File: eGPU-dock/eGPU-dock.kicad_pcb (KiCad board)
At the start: 2 copper layers, 40 parts, among them Y1 25MHz

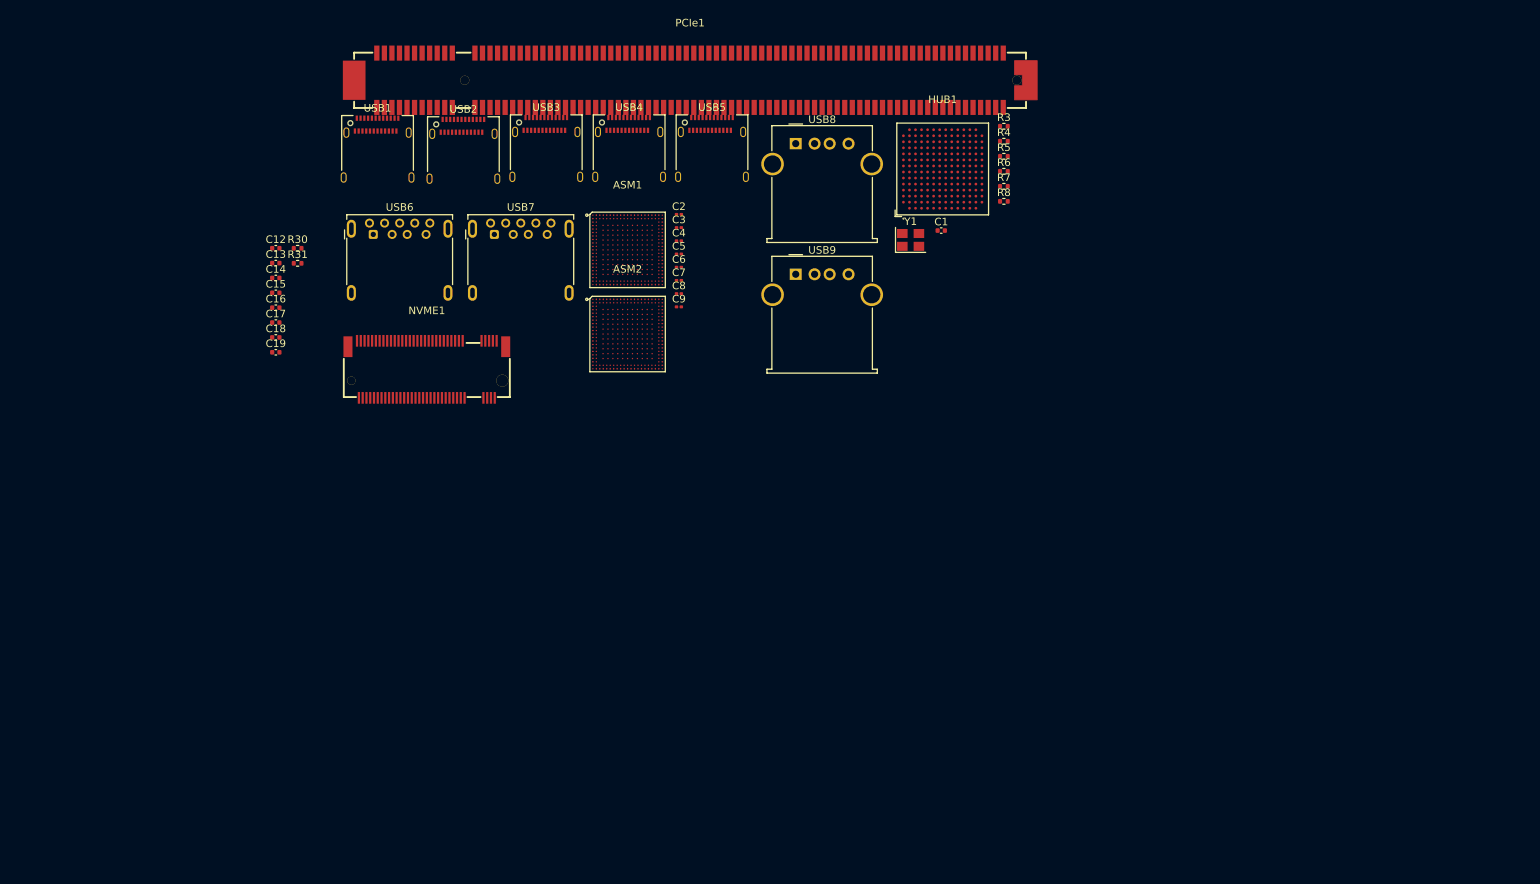
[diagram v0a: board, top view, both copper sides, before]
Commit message: update
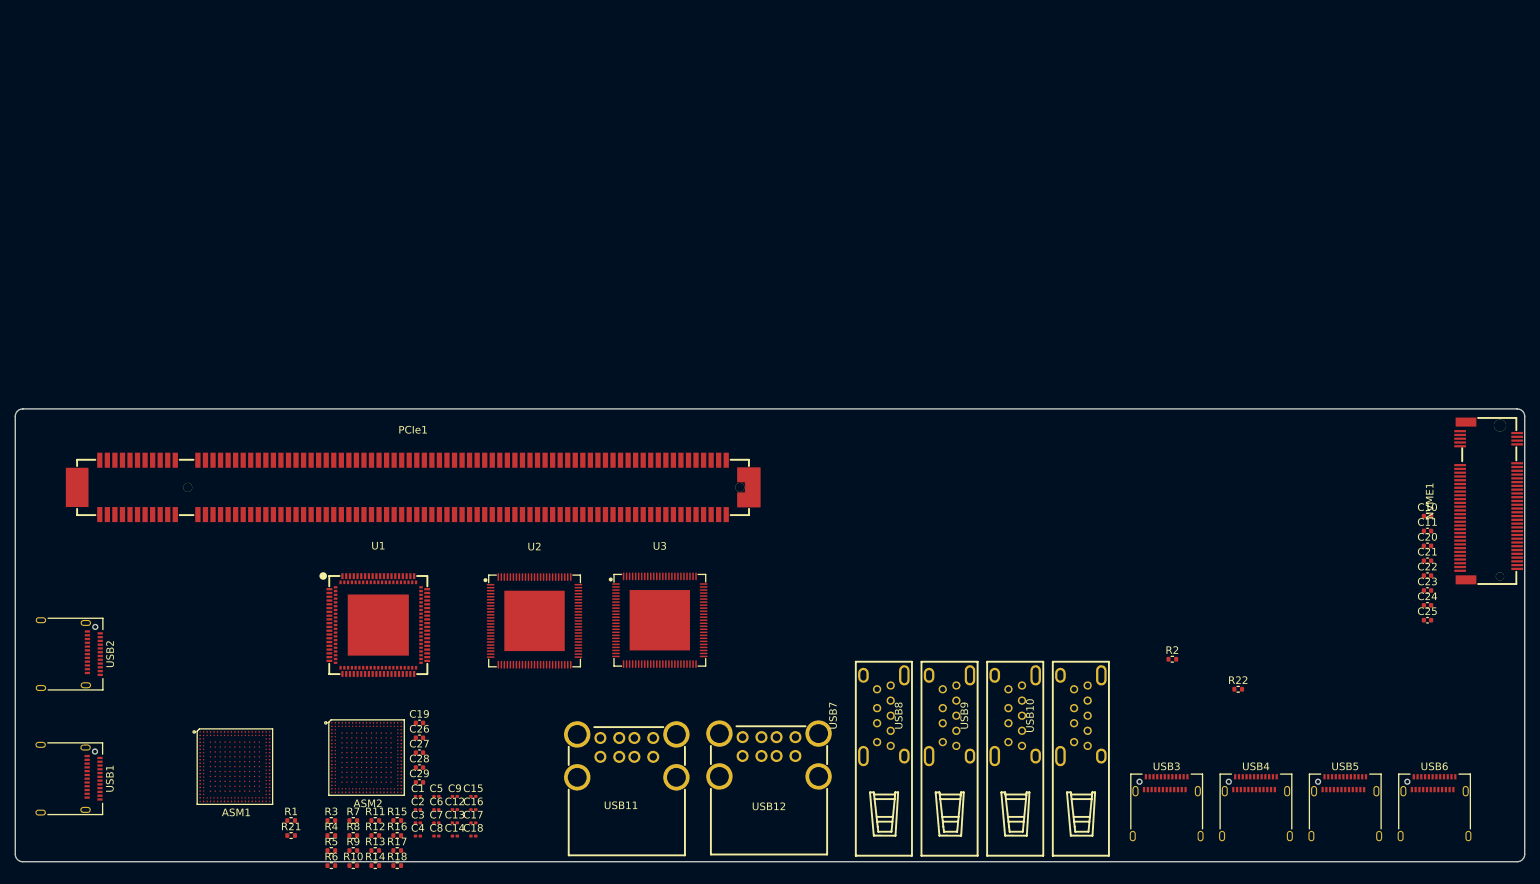
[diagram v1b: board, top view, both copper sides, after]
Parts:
- removed HUB1: CYUSB4347-BZXC, easyeda2kicad:FBGA-192_L12.0-W12.0-P0.80-BL_CY9BF318TBGL-GK7E1
- removed R30, R31: 0Ω, Resistor_SMD:R_0402_1005Metric
- removed Y1: 25MHz, Crystal:Crystal_SMD_3225-4Pin_3.2x2.5mm
- added C10: 0.22u, Capacitor_SMD:C_0402_1005Metric, F.Cu at (237.1, 104.2)
- added C11: 0.22u, Capacitor_SMD:C_0402_1005Metric, F.Cu at (237.1, 106.2)
- added C20: 0.22u, Capacitor_SMD:C_0402_1005Metric, F.Cu at (237.1, 108.2)
- added C21: 0.22u, Capacitor_SMD:C_0402_1005Metric, F.Cu at (237.1, 110.1)
- added C22: 0.22u, Capacitor_SMD:C_0402_1005Metric, F.Cu at (237.1, 112.1)
- added C23: 0.22u, Capacitor_SMD:C_0402_1005Metric, F.Cu at (237.1, 114.1)
- added C24: 0.22u, Capacitor_SMD:C_0402_1005Metric, F.Cu at (237.1, 116.0)
- added C25: 0.22u, Capacitor_SMD:C_0402_1005Metric, F.Cu at (237.1, 118.0)
- added C26: 0.22u, Capacitor_SMD:C_0402_1005Metric, F.Cu at (103.6, 133.6)
- added C27: 0.22u, Capacitor_SMD:C_0402_1005Metric, F.Cu at (103.6, 135.6)
- added C28: 0.22u, Capacitor_SMD:C_0402_1005Metric, F.Cu at (103.6, 137.5)
- added C29: 220p, Capacitor_SMD:C_0402_1005Metric, F.Cu at (103.6, 139.5)
- added R1: 10k, Resistor_SMD:R_0402_1005Metric, F.Cu at (86.5, 144.5)
- added R10: 0Ω, Resistor_SMD:R_0402_1005Metric, F.Cu at (94.8, 150.5)
- added R11: 0Ω, Resistor_SMD:R_0402_1005Metric, F.Cu at (97.7, 144.5)
- added R12: 0Ω, Resistor_SMD:R_0402_1005Metric, F.Cu at (97.7, 146.5)
- added R13: 0Ω, Resistor_SMD:R_0402_1005Metric, F.Cu at (97.7, 148.5)
- added R14: 0Ω, Resistor_SMD:R_0402_1005Metric, F.Cu at (97.7, 150.5)
- added R15: 10k, Resistor_SMD:R_0402_1005Metric, F.Cu at (100.6, 144.5)
- added R16: 10k, Resistor_SMD:R_0402_1005Metric, F.Cu at (100.6, 146.5)
- added R17: 1KΩ, Resistor_SMD:R_0402_1005Metric, F.Cu at (100.6, 148.5)
- added R18: 10KΩ, Resistor_SMD:R_0402_1005Metric, F.Cu at (100.6, 150.5)
- added R2: 0Ω, Resistor_SMD:R_0402_1005Metric, F.Cu at (203.3, 123.2)
- added R21: 10k, Resistor_SMD:R_0402_1005Metric, F.Cu at (86.5, 146.5)
- added R22: 0Ω, Resistor_SMD:R_0402_1005Metric, F.Cu at (212.0, 127.2)
- added R9: 0Ω, Resistor_SMD:R_0402_1005Metric, F.Cu at (94.8, 148.5)
- added U1: PCI11414-I/PMX, easyeda2kicad:QFN-164_L13.0-W13.0-P0.50-TL-EP8.0, F.Cu at (98.1, 118.6)
- added U2: USB7216C/KDX, easyeda2kicad:VQFN-100_L12.0-W12.0-P0.40-TL-EP8.0, F.Cu at (118.8, 118.1)
- added U3: USB7206C-I/KDX, easyeda2kicad:VQFN-100_L12.0-W12.0-P0.40-TL-EP8.0, F.Cu at (135.4, 118.0)
- added USB10: HC-USB3.0-L257-P, easyeda2kicad:USB-3.0-A-TH_HOOYA_USB-303L-L-SU, F.Cu at (191.2, 130.7)
- added USB11: USB-269-BRW, easyeda2kicad:USB-A-TH_USB-269-BRW, F.Cu at (131.0, 136.0)
- added USB12: USB-269-BRW, easyeda2kicad:USB-A-TH_USB-269-BRW, F.Cu at (149.9, 135.9)
- ASM1, ASM2: footprint easyeda2kicad:FCCSP-273_L10.0-W10.0-P0.45-TL -> eGPUlib:ASM2464PDX
- C1: value 10p -> 0.33u; footprint Capacitor_SMD:C_0402_1005Metric -> Capacitor_SMD:C_0201_0603Metric
- C12, C13, C14, C15, C16, C17, C18: value 0.22u -> 0.33u; footprint Capacitor_SMD:C_0402_1005Metric -> Capacitor_SMD:C_0201_0603Metric
- PCIe1: value X1611WVS-164-9TV30 -> PCIexpress_x16
- USB6: value USB3_A -> USB_C_Receptacle; footprint Connector_USB:USB3_A_Molex_48393-001 -> Connector_USB:USB_C_Receptacle_Amphenol_12401610E4-2A
- USB7: value USB3_A -> HC-USB3.0-L257-P; footprint Connector_USB:USB3_A_Molex_48393-001 -> easyeda2kicad:USB-3.0-A-TH_HOOYA_USB-303L-L-SU
- USB8, USB9: value USB_A -> HC-USB3.0-L257-P; footprint Connector_USB:USB_A_Molex_67643_Horizontal -> easyeda2kicad:USB-3.0-A-TH_HOOYA_USB-303L-L-SU
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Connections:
- net /CC1_C renamed /USB4_1_CC1_C
- net /CC2_C renamed /USB4_1_CC2_C
- net /SBU1_C renamed /USB4_1_SBU1_C
- net /SBU2_C renamed /USB4_1_SBU2_C
- net /URX0_C+ renamed /USB4_1_RX0_C+
- net /URX0_C- renamed /USB4_1_RX0_C-
- net /URX1_C+ renamed /USB4_1_RX1_C+
- net /URX1_C- renamed /USB4_1_RX1_C-
- net /USB2_C_D+ renamed /USB4_1_2.0_C_D+
- net /USB2_C_D- renamed /USB4_1_2.0_C_D-
- net /UTX0_C+ renamed /USB4_1_TX0_C+
- net /UTX0_C- renamed /USB4_1_TX0_C-
- net /UTX1_C+ renamed /USB4_1_TX1_C+
- net /UTX1_C- renamed /USB4_1_TX1_C-
- net ActLED1 renamed ASM1_ActLED1
- net ActLED2 renamed ASM1_ActLED2
- net ActLED3 renamed ASM1_ActLED3
- net ActLED4 renamed ASM1_ActLED4
- net CC1 renamed USB4_1_CC1
- net CC2 renamed USB4_1_CC2
- net CLKREQ2# renamed ASM1_CLKREQ2#
- net CLKREQ3# renamed ASM1_CLKREQ3#
- net GPIO1 renamed ASM1_GPIO1
- net GPIO19 renamed ASM1_GPIO19
- net GPIO2 renamed ASM1_GPIO2
- net GPIO20 renamed ASM1_GPIO20
- net GPIO21 renamed ASM1_GPIO21
- net GPIO27 renamed ASM1_GPIO27
- net HDDPC renamed PCIe_HDDPC
- net P1_LED renamed ASM1_P1_LED
- net P2_LED renamed ASM1_P2_LED
- net P3_LED renamed ASM1_P3_LED
- net P4_LED renamed ASM1_P4_LED
- net RST# renamed ASM1_RST#
- net SBU1 renamed USB4_1_SBU1
- net SBU2 renamed USB4_1_SBU2
- net SPI_CLK renamed ASM1_SPI_CLK
- net SPI_CS# renamed ASM1_SPI_CS#
- net SPI_DI renamed ASM1_SPI_DI
- net SPI_DO renamed ASM1_SPI_DO
- net TEST_EN renamed ASM1_TEST_EN
- net UREXT renamed ASM1_UREXT
- net URX0+ renamed USB4_1_RX0+
- net URX0- renamed USB4_1_RX0-
- net URX1+ renamed USB4_1_RX1+
- net URX1- renamed USB4_1_RX1-
- net USB2_D+ renamed USB4_1_2.0_D+
- net USB2_D- renamed USB4_1_2.0_D-
- net UTX0+ renamed USB4_1_TX0+
- net UTX0- renamed USB4_1_TX0-
- net UTX1+ renamed USB4_1_TX1+
- net UTX1- renamed USB4_1_TX1-
- ASM1 pad A13: PE_WAKE# -> ASM1_PE_WAKE#
- ASM1 pad A19: CLKREQ1# -> PCIe_CLKREQ#
- ASM1 pad A20: CLKREQ0# -> ASM1_CLKREQ1#
- ASM1 pad A21: UART_RX -> unconnected-(ASM1B-PRSNT0#/UART_RX-PadA21)
- ASM1 pad AA1: unconnected-(ASM1C-GNDA-PadAA1) -> GNDA
- ASM1 pad AA12: unconnected-(ASM1C-GNDA-PadAA12) -> GNDA
- ASM1 pad AA14: unconnected-(ASM1C-GNDA-PadAA14) -> GNDA
- ASM1 pad AA16: unconnected-(ASM1C-GNDA-PadAA16) -> GNDA
- ASM1 pad AA18: unconnected-(ASM1C-GNDA-PadAA18) -> GNDA
- ASM1 pad AA2: unconnected-(ASM1C-GNDA-PadAA2) -> GNDA
- ASM1 pad AA20: unconnected-(ASM1C-GNDA-PadAA20) -> GNDA
- ASM1 pad AA21: unconnected-(ASM1C-GNDA-PadAA21) -> GNDA
- ASM1 pad AA4: XI -> ASM1_XI
- ASM1 pad AA5: unconnected-(ASM1C-GNDA-PadAA5) -> GNDA
- ASM1 pad AA8: REFCLK+ -> PCIe_REFCLK+
- ASM1 pad AA9: unconnected-(ASM1C-GNDA-PadAA9) -> GNDA
- ASM1 pad B21: UART_TX -> unconnected-(ASM1B-MEMREPAIR/UART_TX-PadB21)
- ASM1 pad D11: unconnected-(ASM1C-GND-PadD11) -> GND
- ASM1 pad D13: unconnected-(ASM1C-VCCH-PadD13) -> +3.3V_LDO
- ASM1 pad D14: unconnected-(ASM1C-VDD-PadD14) -> VDD
- ASM1 pad D16: unconnected-(ASM1C-VDD-PadD16) -> VDD
- ASM1 pad D17: unconnected-(ASM1C-GND-PadD17) -> GND
- ASM1 pad D18: unconnected-(ASM1C-GND-PadD18) -> GND
- ASM1 pad D4: unconnected-(ASM1C-GND-PadD4) -> GND
- ASM1 pad D5: unconnected-(ASM1C-GND-PadD5) -> GND
- ASM1 pad D6: unconnected-(ASM1C-VCCH-PadD6) -> +3.3V_LDO
- ASM1 pad D8: unconnected-(ASM1C-VCCH-PadD8) -> +3.3V_LDO
- ASM1 pad D9: unconnected-(ASM1C-VCCH-PadD9) -> +3.3V_LDO
- ASM1 pad E1: I2C_CLK -> unconnected-(ASM1B-I2C_CLK_P-PadE1)
- ASM1 pad E11: unconnected-(ASM1C-VDD-PadE11) -> VDD
- ASM1 pad E13: unconnected-(ASM1C-VCCH-PadE13) -> +3.3V_LDO
- ASM1 pad E14: unconnected-(ASM1C-VDD-PadE14) -> VDD
- ASM1 pad E16: unconnected-(ASM1C-VDD-PadE16) -> VDD
- ASM1 pad E17: unconnected-(ASM1C-GND-PadE17) -> GND
- ASM1 pad E18: unconnected-(ASM1C-GND-PadE18) -> GND
- ASM1 pad E4: unconnected-(ASM1C-GND-PadE4) -> GND
- ASM1 pad E5: unconnected-(ASM1C-GND-PadE5) -> GND
- ASM1 pad E6: unconnected-(ASM1C-VCCH-PadE6) -> +3.3V_LDO
- ASM1 pad E8: unconnected-(ASM1C-VCCH-PadE8) -> +3.3V_LDO
- ASM1 pad E9: unconnected-(ASM1C-VCCH-PadE9) -> +3.3V_LDO
- ASM1 pad F1: I2C_DATA -> unconnected-(ASM1B-I2C_DATA_P-PadF1)
- ASM1 pad F11: unconnected-(ASM1C-VDD-PadF11) -> VDD
- ASM1 pad F13: unconnected-(ASM1C-VCCH-PadF13) -> +3.3V_LDO
- ASM1 pad F14: unconnected-(ASM1C-VDD-PadF14) -> VDD
- ASM1 pad F16: unconnected-(ASM1C-VDD-PadF16) -> VDD
- ASM1 pad F17: unconnected-(ASM1C-GND-PadF17) -> GND
- ASM1 pad F18: unconnected-(ASM1C-GND-PadF18) -> GND
- ASM1 pad F4: unconnected-(ASM1C-GND-PadF4) -> GND
- ASM1 pad F5: unconnected-(ASM1C-GND-PadF5) -> GND
- ASM1 pad F6: unconnected-(ASM1C-VCCH-PadF6) -> +3.3V_LDO
- ASM1 pad F8: unconnected-(ASM1C-GND-PadF8) -> GND
- ASM1 pad F9: unconnected-(ASM1C-VDD-PadF9) -> VDD
- ASM1 pad G1: VBUS -> ASM1_VBUS
- ASM1 pad G21: PERST0# -> PCIe_PERST0#
- ASM1 pad H11: unconnected-(ASM1C-VDD-PadH11) -> VDD
- ASM1 pad H13: unconnected-(ASM1C-VDD-PadH13) -> VDD
- ASM1 pad H14: unconnected-(ASM1C-VDD-PadH14) -> VDD
- ASM1 pad H16: unconnected-(ASM1C-VDD-PadH16) -> VDD
- ASM1 pad H17: unconnected-(ASM1C-GND-PadH17) -> GND
- ASM1 pad H18: unconnected-(ASM1C-GND-PadH18) -> GND
- ASM1 pad H4: unconnected-(ASM1C-GND-PadH4) -> GND
- ASM1 pad H5: unconnected-(ASM1C-VCCA33-PadH5) -> +3.3VA
- ASM1 pad H6: unconnected-(ASM1C-VCCH-PadH6) -> +3.3V_LDO
- ASM1 pad H8: unconnected-(ASM1C-GND-PadH8) -> GND
- ASM1 pad H9: unconnected-(ASM1C-VDD-PadH9) -> VDD
- ASM1 pad J11: unconnected-(ASM1C-GND-PadJ11) -> GND
- ASM1 pad J13: unconnected-(ASM1C-VDD-PadJ13) -> VDD
- ASM1 pad J14: unconnected-(ASM1C-VDD-PadJ14) -> VDD
- ASM1 pad J16: unconnected-(ASM1C-VDD-PadJ16) -> VDD
- ASM1 pad J17: unconnected-(ASM1C-VDD-PadJ17) -> VDD
- ASM1 pad J18: unconnected-(ASM1C-VDD-PadJ18) -> VDD
- ASM1 pad J20: unconnected-(ASM1C-VDD-PadJ20) -> VDD
- ASM1 pad J21: unconnected-(ASM1C-VDD-PadJ21) -> VDD
- ASM1 pad J4: unconnected-(ASM1C-GND-PadJ4) -> GND
- ASM1 pad J5: unconnected-(ASM1C-GND-PadJ5) -> GND
- ASM1 pad J6: unconnected-(ASM1C-GND-PadJ6) -> GND
- ASM1 pad J8: unconnected-(ASM1C-VDD-PadJ8) -> VDD
- ASM1 pad J9: unconnected-(ASM1C-VDD-PadJ9) -> VDD
- ASM1 pad K2: unconnected-(ASM1C-GND-PadK2) -> GND
- ASM1 pad K20: unconnected-(ASM1C-VDD-PadK20) -> VDD
- ASM1 pad K21: unconnected-(ASM1C-VDD-PadK21) -> VDD
- ASM1 pad L1: unconnected-(ASM1C-GNDA-PadL1) -> GNDA
- ASM1 pad L11: unconnected-(ASM1C-VDD-PadL11) -> VDD
- ASM1 pad L13: unconnected-(ASM1C-GND-PadL13) -> GND
- ASM1 pad L14: unconnected-(ASM1C-VDD-PadL14) -> VDD
- ASM1 pad L16: unconnected-(ASM1C-VCCL-PadL16) -> VCCL
- ASM1 pad L17: unconnected-(ASM1C-VCCL-PadL17) -> VCCL
- ASM1 pad L18: unconnected-(ASM1C-VCCL-PadL18) -> VCCL
- ASM1 pad L2: unconnected-(ASM1C-GNDA-PadL2) -> GNDA
- ASM1 pad L20: unconnected-(ASM1C-VCCL-PadL20) -> VCCL
- ASM1 pad L21: unconnected-(ASM1C-VCCL-PadL21) -> VCCL
- ASM1 pad L4: unconnected-(ASM1C-GNDA-PadL4) -> GNDA
- ASM1 pad L5: unconnected-(ASM1C-GNDA-PadL5) -> GNDA
- ASM1 pad L6: unconnected-(ASM1C-VCCL-PadL6) -> VCCL
- ASM1 pad L8: unconnected-(ASM1C-VDD-PadL8) -> VDD
- ASM1 pad L9: unconnected-(ASM1C-GND-PadL9) -> GND
- ASM1 pad M20: unconnected-(ASM1C-GNDA-PadM20) -> GNDA
- ASM1 pad M21: unconnected-(ASM1C-GNDA-PadM21) -> GNDA
- ASM1 pad N1: unconnected-(ASM1C-GNDA-PadN1) -> GNDA
- ASM1 pad N11: unconnected-(ASM1C-GND-PadN11) -> GND
- ASM1 pad N13: unconnected-(ASM1C-GND-PadN13) -> GND
- ASM1 pad N14: unconnected-(ASM1C-VDD-PadN14) -> VDD
- ASM1 pad N16: unconnected-(ASM1C-VCCL-PadN16) -> VCCL
- ASM1 pad N17: unconnected-(ASM1C-GNDA-PadN17) -> GNDA
- ASM1 pad N18: unconnected-(ASM1C-GNDA-PadN18) -> GNDA
- ASM1 pad N2: unconnected-(ASM1C-GNDA-PadN2) -> GNDA
- ASM1 pad N4: unconnected-(ASM1C-GNDA-PadN4) -> GNDA
- ASM1 pad N5: unconnected-(ASM1C-GNDA-PadN5) -> GNDA
- ASM1 pad N6: unconnected-(ASM1C-VCCL-PadN6) -> VCCL
- ASM1 pad N8: unconnected-(ASM1C-VDD-PadN8) -> VDD
- ASM1 pad N9: unconnected-(ASM1C-GND-PadN9) -> GND
- ASM1 pad P11: unconnected-(ASM1C-GND-PadP11) -> GND
- ASM1 pad P13: unconnected-(ASM1C-VDD-PadP13) -> VDD
- ASM1 pad P14: unconnected-(ASM1C-VDD-PadP14) -> VDD
- ASM1 pad P16: unconnected-(ASM1C-VCCL-PadP16) -> VCCL
- ASM1 pad P17: unconnected-(ASM1C-GNDA-PadP17) -> GNDA
- ASM1 pad P18: unconnected-(ASM1C-GNDA-PadP18) -> GNDA
- ASM1 pad P20: unconnected-(ASM1C-GNDA-PadP20) -> GNDA
- ASM1 pad P21: unconnected-(ASM1C-GNDA-PadP21) -> GNDA
- ASM1 pad P4: unconnected-(ASM1C-GNDA-PadP4) -> GNDA
- ASM1 pad P5: unconnected-(ASM1C-GNDA-PadP5) -> GNDA
- ASM1 pad P6: unconnected-(ASM1C-VCCL-PadP6) -> VCCL
- ASM1 pad P8: unconnected-(ASM1C-VDD-PadP8) -> VDD
- ASM1 pad P9: unconnected-(ASM1C-GND-PadP9) -> GND
- ASM1 pad R1: unconnected-(ASM1C-GNDA-PadR1) -> GNDA
- ASM1 pad R2: unconnected-(ASM1C-GNDA-PadR2) -> GNDA
- ASM1 pad T11: unconnected-(ASM1C-VDD-PadT11) -> VDD
- ASM1 pad T13: unconnected-(ASM1C-VDD-PadT13) -> VDD
- ASM1 pad T14: unconnected-(ASM1C-VDD-PadT14) -> VDD
- ASM1 pad T16: unconnected-(ASM1C-VCCL-PadT16) -> VCCL
- ASM1 pad T17: unconnected-(ASM1C-GNDA-PadT17) -> GNDA
- ASM1 pad T18: unconnected-(ASM1C-GNDA-PadT18) -> GNDA
- ASM1 pad T20: unconnected-(ASM1C-GNDA-PadT20) -> GNDA
- ASM1 pad T21: unconnected-(ASM1C-GNDA-PadT21) -> GNDA
- ASM1 pad T4: unconnected-(ASM1C-GNDA-PadT4) -> GNDA
- ASM1 pad T5: unconnected-(ASM1C-GNDA-PadT5) -> GNDA
- ASM1 pad T6: unconnected-(ASM1C-VCCL-PadT6) -> VCCL
- ASM1 pad T8: unconnected-(ASM1C-VDD-PadT8) -> VDD
- ASM1 pad T9: unconnected-(ASM1C-VDD-PadT9) -> VDD
- ASM1 pad U1: unconnected-(ASM1C-GNDA-PadU1) -> GNDA
- ASM1 pad U11: unconnected-(ASM1C-VCCL-PadU11) -> VCCL
- ASM1 pad U13: unconnected-(ASM1C-VCCL-PadU13) -> VCCL
- ASM1 pad U14: unconnected-(ASM1C-VCCL-PadU14) -> VCCL
- ASM1 pad U16: unconnected-(ASM1C-VCCL-PadU16) -> VCCL
- ASM1 pad U17: unconnected-(ASM1C-GNDA-PadU17) -> GNDA
- ASM1 pad U18: unconnected-(ASM1C-GNDA-PadU18) -> GNDA
- ASM1 pad U2: unconnected-(ASM1C-GNDA-PadU2) -> GNDA
- ASM1 pad U4: unconnected-(ASM1C-GNDA-PadU4) -> GNDA
- ASM1 pad U5: unconnected-(ASM1C-GNDA-PadU5) -> GNDA
- ASM1 pad U6: unconnected-(ASM1C-VCCL-PadU6) -> VCCL
- ASM1 pad U8: unconnected-(ASM1C-VDD-PadU8) -> VDD
- ASM1 pad U9: unconnected-(ASM1C-VDD-PadU9) -> VDD
- ASM1 pad V11: unconnected-(ASM1C-GNDA-PadV11) -> GNDA
- ASM1 pad V13: unconnected-(ASM1C-GNDA-PadV13) -> GNDA
- ASM1 pad V14: unconnected-(ASM1C-GNDA-PadV14) -> GNDA
- ASM1 pad V16: unconnected-(ASM1C-GNDA-PadV16) -> GNDA
- ASM1 pad V17: unconnected-(ASM1C-GNDA-PadV17) -> GNDA
- ASM1 pad V18: unconnected-(ASM1C-GNDA-PadV18) -> GNDA
- ASM1 pad V20: unconnected-(ASM1C-GNDA-PadV20) -> GNDA
- ASM1 pad V21: unconnected-(ASM1C-GNDA-PadV21) -> GNDA
- ASM1 pad V4: unconnected-(ASM1C-GNDA-PadV4) -> GNDA
- ASM1 pad V5: unconnected-(ASM1C-GNDA-PadV5) -> GNDA
- ASM1 pad V6: unconnected-(ASM1C-GNDA-PadV6) -> GNDA
- ASM1 pad V8: unconnected-(ASM1C-GNDA-PadV8) -> GNDA
- ASM1 pad V9: unconnected-(ASM1C-GNDA-PadV9) -> GNDA
- ASM1 pad W1: unconnected-(ASM1C-GNDA-PadW1) -> GNDA
- ASM1 pad W2: unconnected-(ASM1C-GNDA-PadW2) -> GNDA
- ASM1 pad Y12: unconnected-(ASM1C-GNDA-PadY12) -> GNDA
- ASM1 pad Y14: unconnected-(ASM1C-GNDA-PadY14) -> GNDA
- ASM1 pad Y16: unconnected-(ASM1C-GNDA-PadY16) -> GNDA
- ASM1 pad Y18: unconnected-(ASM1C-GNDA-PadY18) -> GNDA
- ASM1 pad Y20: unconnected-(ASM1C-GNDA-PadY20) -> GNDA
- ASM1 pad Y21: unconnected-(ASM1C-GNDA-PadY21) -> GNDA
- ASM1 pad Y3: unconnected-(ASM1C-GNDA-PadY3) -> GNDA
- ASM1 pad Y4: XO -> ASM1_XO
- ASM1 pad Y5: unconnected-(ASM1C-GNDA-PadY5) -> GNDA
- ASM1 pad Y8: REFCLK- -> PCIe_REFCLK-
- ASM1 pad Y9: unconnected-(ASM1C-GNDA-PadY9) -> GNDA
- ASM2 pad A1: unconnected-(ASM2A-GPIO3-PadA1) -> ASM2_ActLED2
- ASM2 pad A10: unconnected-(ASM2A-GPIO19-PadA10) -> ASM2_GPIO19
- ASM2 pad A11: unconnected-(ASM2A-GPIO20-PadA11) -> ASM2_GPIO20
- ASM2 pad A12: unconnected-(ASM2A-GPIO21-PadA12) -> ASM2_GPIO21
- ASM2 pad A13: unconnected-(ASM2A-GPIO22-PadA13) -> ASM2_PE_WAKE#
- ASM2 pad A14: unconnected-(ASM2A-GPIO23-PadA14) -> ASM2_CLKREQ2#
- ASM2 pad A15: unconnected-(ASM2A-GPIO24-PadA15) -> ASM2_CLKREQ3#
- ASM2 pad A16: unconnected-(ASM2A-GPIO25-PadA16) -> ASM2_ActLED3
- ASM2 pad A17: unconnected-(ASM2A-GPIO26-PadA17) -> ASM2_ActLED4
- ASM2 pad A18: unconnected-(ASM2A-GPIO27-PadA18) -> ASM2_GPIO27
- ASM2 pad A19: unconnected-(ASM2A-GPIO8-PadA19) -> M.2_CLKREQ#
- ASM2 pad A2: unconnected-(ASM2A-SPI_CS#-PadA2) -> ASM2_SPI_CS#
- ASM2 pad A20: unconnected-(ASM2A-GPIO14-PadA20) -> SW_CLKREQ#
- ASM2 pad A3: unconnected-(ASM2A-SPI_DO-PadA3) -> ASM2_SPI_DO
- ASM2 pad A4: unconnected-(ASM2A-SPI_DI-PadA4) -> ASM2_SPI_DI
- ASM2 pad A5: unconnected-(ASM2A-SPI_CLK-PadA5) -> ASM2_SPI_CLK
- ASM2 pad A6: unconnected-(ASM2A-GPIO15-PadA6) -> ASM2_P1_LED
- ASM2 pad A7: unconnected-(ASM2A-GPIO16-PadA7) -> ASM2_P2_LED
- ASM2 pad A8: unconnected-(ASM2A-GPIO17-PadA8) -> ASM2_P3_LED
- ASM2 pad A9: unconnected-(ASM2A-GPIO18-PadA9) -> ASM2_P4_LED
- ASM2 pad AA1: unconnected-(ASM2C-GNDA-PadAA1) -> GNDA
- ASM2 pad AA10: unconnected-(ASM2B-NC-PadAA10) -> SW_REFCLK+
- ASM2 pad AA12: unconnected-(ASM2C-GNDA-PadAA12) -> GNDA
- ASM2 pad AA13: unconnected-(ASM2A-PRXP3-PadAA13) -> SW_RX1+
- ASM2 pad AA14: unconnected-(ASM2C-GNDA-PadAA14) -> GNDA
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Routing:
- added copper zone on In1.Cu, net GND
- added copper zone on In10.Cu, net GND
- added copper zone on In3.Cu, net GND
- added copper zone on In6.Cu, net GND
- added copper zone on In8.Cu, net GND
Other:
- board outline added: 200 x 60 mm
- copper layers 2 -> 16

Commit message: masive schamatic update
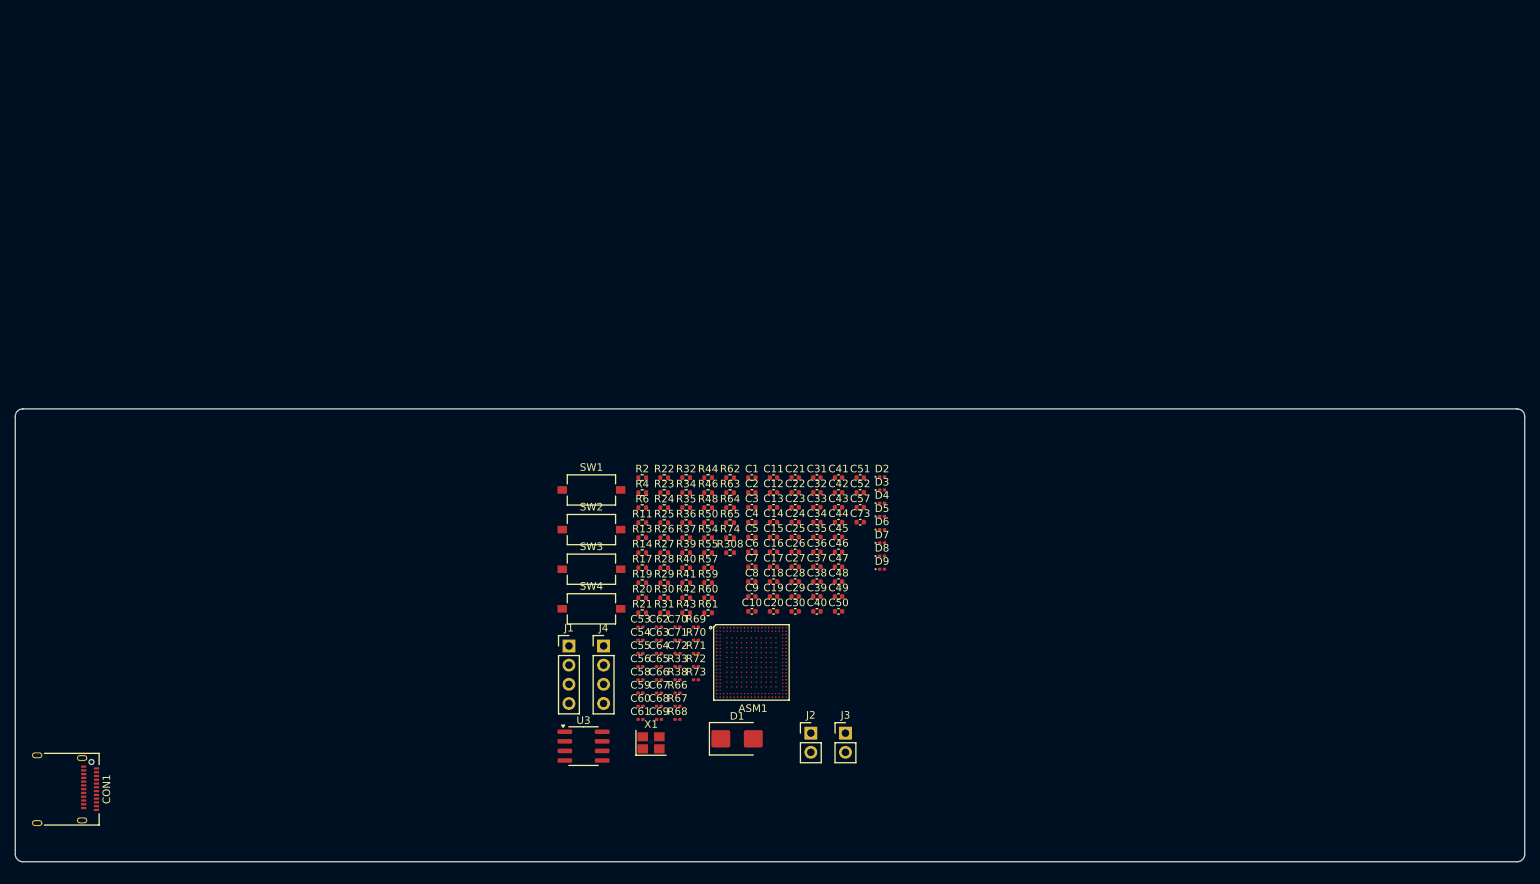
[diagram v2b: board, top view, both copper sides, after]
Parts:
- removed ASM2: ~, eGPUlib:ASM2464PDX
- removed NVME1: AS0BC21-S40BM-7H, easyeda2kicad:CONN-SMD_AS0BC21-S40BM-7H
- removed PCIe1: PCIexpress_x16, easyeda2kicad:CONN-SMD_164P-P1.00_X1611WVS-164-9TV30
- removed R1, R15, R16: 10k, Resistor_SMD:R_0402_1005Metric
- removed R10, R12, R3, R5, R7, R8, R9: 0Ω, Resistor_SMD:R_0402_1005Metric
- removed R18: 10KΩ, Resistor_SMD:R_0402_1005Metric
- removed U1: PCI11414-I/PMX, easyeda2kicad:QFN-164_L13.0-W13.0-P0.50-TL-EP8.0
- removed U2: USB7216C/KDX, easyeda2kicad:VQFN-100_L12.0-W12.0-P0.40-TL-EP8.0
- removed USB1, USB2, USB3, USB4, USB5, USB6: USB_C_Receptacle, Connector_USB:USB_C_Receptacle_Amphenol_12401610E4-2A
- removed USB10, USB7, USB8, USB9: HC-USB3.0-L257-P, easyeda2kicad:USB-3.0-A-TH_HOOYA_USB-303L-L-SU
- removed USB11, USB12: USB-269-BRW, easyeda2kicad:USB-A-TH_USB-269-BRW
- added C30: 0.22UF/10V, Capacitor_SMD:C_0402_1005Metric, F.Cu at (153.3, 116.8)
- added C31: 0.22UF/10V, Capacitor_SMD:C_0402_1005Metric, F.Cu at (156.2, 99.1)
- added C32: 0.22UF/6.3V, Capacitor_SMD:C_0402_1005Metric, F.Cu at (156.2, 101.1)
- added C33: 0.22UF/6.3V, Capacitor_SMD:C_0402_1005Metric, F.Cu at (156.2, 103.0)
- added C34: 0.22UF/10V, Capacitor_SMD:C_0402_1005Metric, F.Cu at (156.2, 105.0)
- added C35: 0.22UF/10V, Capacitor_SMD:C_0402_1005Metric, F.Cu at (156.2, 107.0)
- added C36: 0.22UF/6.3V, Capacitor_SMD:C_0402_1005Metric, F.Cu at (156.2, 109.0)
- added C37: 0.22UF/6.3V, Capacitor_SMD:C_0402_1005Metric, F.Cu at (156.2, 110.9)
- added C38: 10PF/50V, Capacitor_SMD:C_0402_1005Metric, F.Cu at (156.2, 112.9)
- added C39: 0.22UF/10V, Capacitor_SMD:C_0402_1005Metric, F.Cu at (156.2, 114.9)
- added C40: 0.22UF/6.3V, Capacitor_SMD:C_0402_1005Metric, F.Cu at (156.2, 116.8)
- added C41: 0.22UF/6.3V, Capacitor_SMD:C_0402_1005Metric, F.Cu at (159.1, 99.1)
- added C42: 0.22UF/6.3V, Capacitor_SMD:C_0402_1005Metric, F.Cu at (159.1, 101.1)
- added C43: 0.22UF/6.3V, Capacitor_SMD:C_0402_1005Metric, F.Cu at (159.1, 103.0)
- added C44: 0.22UF/6.3V, Capacitor_SMD:C_0402_1005Metric, F.Cu at (159.1, 105.0)
- added C45: 0.22UF/6.3V, Capacitor_SMD:C_0402_1005Metric, F.Cu at (159.1, 107.0)
- added C46: 0.22UF/6.3V, Capacitor_SMD:C_0402_1005Metric, F.Cu at (159.1, 109.0)
- added C47: 0.22UF/16V, Capacitor_SMD:C_0402_1005Metric, F.Cu at (159.1, 110.9)
- added C48: 0.22UF/16V, Capacitor_SMD:C_0402_1005Metric, F.Cu at (159.1, 112.9)
- added C49: 1UF/10V, Capacitor_SMD:C_0402_1005Metric, F.Cu at (159.1, 114.9)
- added C50: 1UF/10V, Capacitor_SMD:C_0402_1005Metric, F.Cu at (159.1, 116.8)
- added C51: 1UF/10V, Capacitor_SMD:C_0402_1005Metric, F.Cu at (161.9, 99.1)
- added C52: 1UF/10V, Capacitor_SMD:C_0402_1005Metric, F.Cu at (161.9, 101.1)
- added C53: 220PF/50V, Capacitor_SMD:C_0201_0603Metric, F.Cu at (132.8, 118.9)
- added C54: 220PF/50V, Capacitor_SMD:C_0201_0603Metric, F.Cu at (132.8, 120.6)
- added C55: 0.1UF/25V, Capacitor_SMD:C_0201_0603Metric, F.Cu at (132.8, 122.4)
- added C56: 0.1UF/25V, Capacitor_SMD:C_0201_0603Metric, F.Cu at (132.8, 124.1)
- added C57: 0.1UF/16V, Capacitor_SMD:C_0402_1005Metric, F.Cu at (161.9, 103.0)
- added C58: 0.1UF/25V, Capacitor_SMD:C_0201_0603Metric, F.Cu at (132.8, 125.9)
- added C59: 0.1UF/25V, Capacitor_SMD:C_0201_0603Metric, F.Cu at (132.8, 127.6)
- added C60: 0.1UF/25V, Capacitor_SMD:C_0201_0603Metric, F.Cu at (132.8, 129.4)
- added C61: 0.1UF/25V, Capacitor_SMD:C_0201_0603Metric, F.Cu at (132.8, 131.1)
- added C62: 0.33UF/25V, Capacitor_SMD:C_0201_0603Metric, F.Cu at (135.3, 118.9)
- added C63: 0.33UF/25V, Capacitor_SMD:C_0201_0603Metric, F.Cu at (135.3, 120.6)
- added C64: 0.33UF/25V, Capacitor_SMD:C_0201_0603Metric, F.Cu at (135.3, 122.4)
- added C65: 0.33UF/25V, Capacitor_SMD:C_0201_0603Metric, F.Cu at (135.3, 124.1)
- added C66: 0.1UF/16V, Capacitor_SMD:C_0201_0603Metric, F.Cu at (135.3, 125.9)
- added C67: 0.1UF/16V, Capacitor_SMD:C_0201_0603Metric, F.Cu at (135.3, 127.6)
- added C68: 1UF/16V, Capacitor_SMD:C_0201_0603Metric, F.Cu at (135.3, 129.4)
- added C69: 0.33UF/25V, Capacitor_SMD:C_0201_0603Metric, F.Cu at (135.3, 131.1)
- added C70: 0.33UF/25V, Capacitor_SMD:C_0201_0603Metric, F.Cu at (137.7, 118.9)
- added C71: 0.33UF/25V, Capacitor_SMD:C_0201_0603Metric, F.Cu at (137.7, 120.6)
- added C72: 0.33UF/25V, Capacitor_SMD:C_0201_0603Metric, F.Cu at (137.7, 122.4)
- added C73: 0.1UF/16V, Capacitor_SMD:C_0402_1005Metric, F.Cu at (161.9, 105.0)
- added CON1: USB_C_Plug, Connector_USB:USB_C_Receptacle_Amphenol_12401610E4-2A, F.Cu at (55.7, 140.4)
- added D1: SR34, Diode_SMD:D_SMB, F.Cu at (145.6, 133.7)
- added D2: ESD150, Diode_SMD:D_0201_0603Metric, F.Cu at (164.8, 99.0)
- added D3: ESD150, Diode_SMD:D_0201_0603Metric, F.Cu at (164.8, 100.7)
- added D4: ESD150, Diode_SMD:D_0201_0603Metric, F.Cu at (164.8, 102.5)
- added D5: ESD150, Diode_SMD:D_0201_0603Metric, F.Cu at (164.8, 104.2)
- added D6: ESD150, Diode_SMD:D_0201_0603Metric, F.Cu at (164.8, 106.0)
- added D7: ESD150, Diode_SMD:D_0201_0603Metric, F.Cu at (164.8, 107.7)
- added D8: ESD150, Diode_SMD:D_0201_0603Metric, F.Cu at (164.8, 109.5)
- added D9: ESD150, Diode_SMD:D_0201_0603Metric, F.Cu at (164.8, 111.2)
- added J1: Conn_01x04, Connector_PinHeader_2.54mm:PinHeader_1x04_P2.54mm_Vertical, F.Cu at (123.4, 121.4)
- added J2: Conn_01x02, Connector_PinHeader_2.54mm:PinHeader_1x02_P2.54mm_Vertical, F.Cu at (155.4, 133.0)
- added J3: Conn_01x02, Connector_PinHeader_2.54mm:PinHeader_1x02_P2.54mm_Vertical, F.Cu at (160.0, 133.0)
- added J4: Conn_01x04, Connector_PinHeader_2.54mm:PinHeader_1x04_P2.54mm_Vertical, F.Cu at (128.0, 121.4)
- added R19: 0Ω, Resistor_SMD:R_0402_1005Metric, F.Cu at (133.1, 113.0)
- added R20: 100KΩ, Resistor_SMD:R_0402_1005Metric, F.Cu at (133.1, 115.0)
- added R23: 1KΩ, Resistor_SMD:R_0402_1005Metric, F.Cu at (136.0, 101.1)
- added R24: 100KΩ, Resistor_SMD:R_0402_1005Metric, F.Cu at (136.0, 103.1)
- added R25: 0Ω, Resistor_SMD:R_0402_1005Metric, F.Cu at (136.0, 105.1)
- added R26: 0Ω, Resistor_SMD:R_0402_1005Metric, F.Cu at (136.0, 107.1)
- added R27: 100KΩ, Resistor_SMD:R_0402_1005Metric, F.Cu at (136.0, 109.1)
- added R28: 100KΩ, Resistor_SMD:R_0402_1005Metric, F.Cu at (136.0, 111.0)
- added R29: 0Ω, Resistor_SMD:R_0402_1005Metric, F.Cu at (136.0, 113.0)
- added R30: 100KΩ, Resistor_SMD:R_0402_1005Metric, F.Cu at (136.0, 115.0)
- added R308: 0Ω, Resistor_SMD:R_0402_1005Metric, F.Cu at (144.7, 109.1)
- added R31: 0Ω, Resistor_SMD:R_0402_1005Metric, F.Cu at (136.0, 117.0)
- added R32: 0Ω, Resistor_SMD:R_0402_1005Metric, F.Cu at (138.9, 99.1)
- added R33: 0Ω, Resistor_SMD:R_0201_0603Metric, F.Cu at (137.7, 124.1)
- added R34: 0Ω, Resistor_SMD:R_0402_1005Metric, F.Cu at (138.9, 101.1)
- added R35: 1KΩ, Resistor_SMD:R_0402_1005Metric, F.Cu at (138.9, 103.1)
- added R36: 0Ω, Resistor_SMD:R_0402_1005Metric, F.Cu at (138.9, 105.1)
- added R37: 0Ω, Resistor_SMD:R_0402_1005Metric, F.Cu at (138.9, 107.1)
- added R38: 0Ω, Resistor_SMD:R_0201_0603Metric, F.Cu at (137.7, 125.9)
- added R39: 2MΩ, Resistor_SMD:R_0402_1005Metric, F.Cu at (138.9, 109.1)
- added R40: 2MΩ, Resistor_SMD:R_0402_1005Metric, F.Cu at (138.9, 111.0)
- added R41: 0Ω, Resistor_SMD:R_0402_1005Metric, F.Cu at (138.9, 113.0)
- added R42: 12.1KΩ, Resistor_SMD:R_0402_1005Metric, F.Cu at (138.9, 115.0)
- added R43: 4.7KΩ, Resistor_SMD:R_0402_1005Metric, F.Cu at (138.9, 117.0)
- added R44: 4.7KΩ, Resistor_SMD:R_0402_1005Metric, F.Cu at (141.8, 99.1)
- added R46: 4.7KΩ, Resistor_SMD:R_0402_1005Metric, F.Cu at (141.8, 101.1)
- added R48: 4.7KΩ, Resistor_SMD:R_0402_1005Metric, F.Cu at (141.8, 103.1)
- added R50: 4.7KΩ, Resistor_SMD:R_0402_1005Metric, F.Cu at (141.8, 105.1)
- added R54: 0Ω, Resistor_SMD:R_0402_1005Metric, F.Cu at (141.8, 107.1)
- added R55: 0Ω, Resistor_SMD:R_0402_1005Metric, F.Cu at (141.8, 109.1)
- added R57: 4.7KΩ, Resistor_SMD:R_0402_1005Metric, F.Cu at (141.8, 111.0)
- added R59: 0Ω, Resistor_SMD:R_0402_1005Metric, F.Cu at (141.8, 113.0)
- added R60: 10KΩ, Resistor_SMD:R_0402_1005Metric, F.Cu at (141.8, 115.0)
- added R61: 4.7KΩ, Resistor_SMD:R_0402_1005Metric, F.Cu at (141.8, 117.0)
- added R62: 4.7KΩ, Resistor_SMD:R_0402_1005Metric, F.Cu at (144.7, 99.1)
- added R63: 0Ω, Resistor_SMD:R_0402_1005Metric, F.Cu at (144.7, 101.1)
- added R64: 0Ω, Resistor_SMD:R_0402_1005Metric, F.Cu at (144.7, 103.1)
- added R65: 0Ω, Resistor_SMD:R_0402_1005Metric, F.Cu at (144.7, 105.1)
- added R66: 220KΩ, Resistor_SMD:R_0201_0603Metric, F.Cu at (137.7, 127.6)
- added R67: 220KΩ, Resistor_SMD:R_0201_0603Metric, F.Cu at (137.7, 129.4)
- added R68: 220KΩ, Resistor_SMD:R_0201_0603Metric, F.Cu at (137.7, 131.1)
- added R69: 220KΩ, Resistor_SMD:R_0201_0603Metric, F.Cu at (140.2, 118.9)
- added R70: 220KΩ, Resistor_SMD:R_0201_0603Metric, F.Cu at (140.2, 120.6)
- added R71: 220KΩ, Resistor_SMD:R_0201_0603Metric, F.Cu at (140.2, 122.4)
- added R72: 220KΩ, Resistor_SMD:R_0201_0603Metric, F.Cu at (140.2, 124.1)
- added R73: 220KΩ, Resistor_SMD:R_0201_0603Metric, F.Cu at (140.2, 125.9)
- added R74: 0Ω, Resistor_SMD:R_0402_1005Metric, F.Cu at (144.7, 107.1)
- added SW1: SW_Push, Button_Switch_SMD:SW_Tactile_SPST_NO_Straight_CK_PTS636Sx25SMTRLFS, F.Cu at (126.3, 100.7)
- added SW2: SW_Push, Button_Switch_SMD:SW_Tactile_SPST_NO_Straight_CK_PTS636Sx25SMTRLFS, F.Cu at (126.3, 106.0)
- added SW3: SW_Push, Button_Switch_SMD:SW_Tactile_SPST_NO_Straight_CK_PTS636Sx25SMTRLFS, F.Cu at (126.3, 111.2)
- added SW4: SW_Push, Button_Switch_SMD:SW_Tactile_SPST_NO_Straight_CK_PTS636Sx25SMTRLFS, F.Cu at (126.3, 116.5)
- added X1: 25 Mhz, Crystal:Crystal_SMD_Abracon_ABM8AIG-4Pin_3.2x2.5mm, F.Cu at (134.2, 134.2)
- C1, C15, C16, C17, C2, C3, C9: value 0.33u -> 2.2UF/6.3V; footprint Capacitor_SMD:C_0201_0603Metric -> Capacitor_SMD:C_0402_1005Metric
- C10, C11: value 0.22u -> 2.2UF/6.3V
- C12, C13, C14, C18, C4, C5, C6: value 0.33u -> 10UF/6.3V; footprint Capacitor_SMD:C_0201_0603Metric -> Capacitor_SMD:C_0402_1005Metric
- C19, C20, C21: value 0.22u -> 10UF/6.3V
- C22, C24, C25, C28: value 0.22u -> 0.22UF/6.3V
- C23, C26, C27: value 0.22u -> 0.22UF/10V
- C29: value 220p -> 0.22UF/6.3V
- C7: value 0.33u -> 22UF/6.3V; footprint Capacitor_SMD:C_0201_0603Metric -> Capacitor_SMD:C_0402_1005Metric
- C8: value 0.33u -> 0.22UF/10V; footprint Capacitor_SMD:C_0201_0603Metric -> Capacitor_SMD:C_0402_1005Metric
- R13: value 0Ω -> 4.7KΩ
- R14, R22: value 0Ω -> 1KΩ
- R17: value 1KΩ -> 0Ω
- R2: value 0Ω -> 20Ω
- R21: value 10k -> 100KΩ
- R6: value 0Ω -> 100KΩ
- U3: value USB7206C-I/KDX -> W25X20CLSN; footprint easyeda2kicad:VQFN-100_L12.0-W12.0-P0.40-TL-EP8.0 -> Package_SO:SOIC-8_3.9x4.9mm_P1.27mm
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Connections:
- net ASM1_ActLED3 renamed GPIO25
- net ASM1_ActLED4 renamed GPIO26
- net ASM1_CLKREQ1# renamed GPIO14
- net ASM1_CLKREQ2# renamed GPIO23
- net ASM1_CLKREQ3# renamed GPIO24
- net ASM1_GPIO19 renamed GPIO19
- net ASM1_GPIO20 renamed GPIO20
- net ASM1_GPIO21 renamed GPIO21
- net ASM1_P1_LED renamed P1_LED
- net ASM1_P2_LED renamed P2_LED
- net ASM1_P3_LED renamed P3_LED
- net ASM1_P4_LED renamed P4_LED
- net ASM1_XI renamed X1
- ASM1 pad A1: ASM1_ActLED2 -> GPIO3
- ASM1 pad A13: ASM1_PE_WAKE# -> GPIO22
- ASM1 pad A18: ASM1_GPIO27 -> GPIO27
- ASM1 pad A19: PCIe_CLKREQ# -> GPIO8
- ASM1 pad A2: ASM1_SPI_CS# -> SPI_CS#
- ASM1 pad A21: unconnected-(ASM1B-PRSNT0#/UART_RX-PadA21) -> UART_RX
- ASM1 pad A3: ASM1_SPI_DO -> SPI_DO
- ASM1 pad A4: ASM1_SPI_DI -> SPI_DI
- ASM1 pad A5: ASM1_SPI_CLK -> SPI_CLK
- ASM1 pad AA1: GNDA -> GND
- ASM1 pad AA10: unconnected-(ASM1A-NC/REFCLKP2-PadAA10) -> REFCLK2+
- ASM1 pad AA11: unconnected-(ASM1A-NC/REFCLKP1-PadAA11) -> REFCLK1+
- ASM1 pad AA12: GNDA -> GND
- ASM1 pad AA13: PCIe_RX3+ -> PRX3+
- ASM1 pad AA14: GNDA -> GND
- ASM1 pad AA15: PCIe_TX3- -> PTX3-
- ASM1 pad AA16: GNDA -> GND
- ASM1 pad AA17: PCIe_TX2- -> PTX2-
- ASM1 pad AA18: GNDA -> GND
- ASM1 pad AA19: PCIe_RX2- -> PRX2-
- ASM1 pad AA2: GNDA -> GND
- ASM1 pad AA20: GNDA -> GND
- ASM1 pad AA21: GNDA -> GND
- ASM1 pad AA3: ASM1_UREXT -> UREXT
- ASM1 pad AA5: GNDA -> GND
- ASM1 pad AA6: USB4_1_CC1 -> CC1
- ASM1 pad AA7: unconnected-(ASM1A-NC/REFCLKP3-PadAA7) -> REFCLK3+
- ASM1 pad AA8: PCIe_REFCLK+ -> REFCLK0+
- ASM1 pad AA9: GNDA -> GND
- ASM1 pad B1: ASM1_GPIO2 -> GPIO2
- ASM1 pad B21: unconnected-(ASM1B-MEMREPAIR/UART_TX-PadB21) -> UART_TX
- ASM1 pad C1: ASM1_GPIO1 -> GPIO1
- ASM1 pad C21: PCIe_HDDPC -> HDDPC
- ASM1 pad D1: ASM1_ActLED1 -> GPIO0
- ASM1 pad D13: +3.3V_LDO -> unconnected-(ASM1E-VCCH-PadD13)
- ASM1 pad D14: VDD -> VDD095
- ASM1 pad D16: VDD -> VDD095
- ASM1 pad D21: unconnected-(ASM1A-NC/PERST3#-PadD21) -> PERST_B3
- ASM1 pad D6: +3.3V_LDO -> unconnected-(ASM1E-VCCH-PadD6)
- ASM1 pad D8: +3.3V_LDO -> unconnected-(ASM1E-VCCH-PadD8)
- ASM1 pad D9: +3.3V_LDO -> unconnected-(ASM1E-VCCH-PadD9)
- ASM1 pad E1: unconnected-(ASM1B-I2C_CLK_P-PadE1) -> I2C_CLK_PD
- ASM1 pad E11: VDD -> VDD095
- ASM1 pad E13: +3.3V_LDO -> unconnected-(ASM1E-VCCH-PadE13)
- ASM1 pad E14: VDD -> VDD095
- ASM1 pad E16: VDD -> VDD095
- ASM1 pad E21: unconnected-(ASM1A-NC/PERST2#-PadE21) -> PERST_B2
- ASM1 pad E6: +3.3V_LDO -> unconnected-(ASM1E-VCCH-PadE6)
- ASM1 pad E8: +3.3V_LDO -> unconnected-(ASM1E-VCCH-PadE8)
- ASM1 pad E9: +3.3V_LDO -> unconnected-(ASM1E-VCCH-PadE9)
- ASM1 pad F1: unconnected-(ASM1B-I2C_DATA_P-PadF1) -> I2C_DATA_PD
- ASM1 pad F11: VDD -> VDD095
- ASM1 pad F13: +3.3V_LDO -> unconnected-(ASM1E-VCCH-PadF13)
- ASM1 pad F14: VDD -> VDD095
- ASM1 pad F16: VDD -> VDD095
- ASM1 pad F21: unconnected-(ASM1A-NC/PERST1#-PadF21) -> PERST_B1
- ASM1 pad F6: +3.3V_LDO -> unconnected-(ASM1E-VCCH-PadF6)
- ASM1 pad F9: VDD -> VDD095
- ASM1 pad G1: ASM1_VBUS -> VBUS
- ASM1 pad G21: PCIe_PERST0# -> PERST_B
- ASM1 pad H1: ASM1_RST# -> RST
- ASM1 pad H11: VDD -> VDD095
- ASM1 pad H13: VDD -> VDD095
- ASM1 pad H14: VDD -> VDD095
- ASM1 pad H16: VDD -> VDD095
- ASM1 pad H21: ASM1_TEST_EN -> TEST_EN
- ASM1 pad H5: +3.3VA -> unconnected-(ASM1E-VCCA33-PadH5)
- ASM1 pad H6: +3.3V_LDO -> unconnected-(ASM1E-VCCH-PadH6)
- ASM1 pad H9: VDD -> VDD095
- ASM1 pad J1: USB4_1_SBU2 -> SBU2
- ASM1 pad J13: VDD -> VDD095
- ASM1 pad J14: VDD -> VDD095
- ASM1 pad J16: VDD -> VDD095
- ASM1 pad J17: VDD -> VDD095
- ASM1 pad J18: VDD -> VDD095
- ASM1 pad J20: VDD -> VDD095
- ASM1 pad J21: VDD -> VDD095
- ASM1 pad J8: VDD -> VDD095
- ASM1 pad J9: VDD -> VDD095
- ASM1 pad K1: USB4_1_SBU1 -> SBU1
- ASM1 pad K20: VDD -> VDD095
- ASM1 pad K21: VDD -> VDD095
- ASM1 pad L1: GNDA -> GND
- ASM1 pad L11: VDD -> VDD095
- ASM1 pad L14: VDD -> VDD095
- ASM1 pad L16: VCCL -> unconnected-(ASM1E-VCCL-PadL16)
- ASM1 pad L17: VCCL -> unconnected-(ASM1E-VCCL-PadL17)
- ASM1 pad L18: VCCL -> unconnected-(ASM1E-VCCL-PadL18)
- ASM1 pad L2: GNDA -> GND
- ASM1 pad L20: VCCL -> unconnected-(ASM1E-VCCL-PadL20)
- ASM1 pad L21: VCCL -> unconnected-(ASM1E-VCCL-PadL21)
- ASM1 pad L4: GNDA -> GND
- ASM1 pad L5: GNDA -> GND
- ASM1 pad L6: VCCL -> unconnected-(ASM1E-VCCL-PadL6)
- ASM1 pad L8: VDD -> VDD095
- ASM1 pad M1: USB4_1_2.0_D+ -> UD+
- ASM1 pad M2: USB4_1_2.0_D- -> UD-
- ASM1 pad M20: GNDA -> GND
- ASM1 pad M21: GNDA -> GND
- ASM1 pad N1: GNDA -> GND
- ASM1 pad N14: VDD -> VDD095
- ASM1 pad N16: VCCL -> unconnected-(ASM1E-VCCL-PadN16)
- ASM1 pad N17: GNDA -> GND
- ASM1 pad N18: GNDA -> GND
- ASM1 pad N2: GNDA -> GND
- ASM1 pad N20: PCIe_RX0- -> PRX0-
- ASM1 pad N21: PCIe_RX0+ -> PRX0+
- ASM1 pad N4: GNDA -> GND
- ASM1 pad N5: GNDA -> GND
- ASM1 pad N6: VCCL -> unconnected-(ASM1E-VCCL-PadN6)
- ASM1 pad N8: VDD -> VDD095
- ASM1 pad P1: USB4_1_RX0+ -> URX0+
- ASM1 pad P13: VDD -> VDD095
- ASM1 pad P14: VDD -> VDD095
- ASM1 pad P16: VCCL -> unconnected-(ASM1E-VCCL-PadP16)
- ASM1 pad P17: GNDA -> GND
- ASM1 pad P18: GNDA -> GND
- ASM1 pad P2: USB4_1_RX0- -> URX0-
- ASM1 pad P20: GNDA -> GND
- ASM1 pad P21: GNDA -> GND
- ASM1 pad P4: GNDA -> GND
- ASM1 pad P5: GNDA -> GND
- ASM1 pad P6: VCCL -> unconnected-(ASM1E-VCCL-PadP6)
- ASM1 pad P8: VDD -> VDD095
- ASM1 pad R1: GNDA -> GND
- ASM1 pad R2: GNDA -> GND
- ASM1 pad R20: PCIe_TX0+ -> PTX0+
- ASM1 pad R21: PCIe_TX0- -> PTX0-
- ASM1 pad T1: USB4_1_TX0+ -> UTX0+
- ASM1 pad T11: VDD -> VDD095
- ASM1 pad T13: VDD -> VDD095
- ASM1 pad T14: VDD -> VDD095
- ASM1 pad T16: VCCL -> unconnected-(ASM1E-VCCL-PadT16)
- ASM1 pad T17: GNDA -> GND
- ASM1 pad T18: GNDA -> GND
- ASM1 pad T2: USB4_1_TX0- -> UTX0-
- ASM1 pad T20: GNDA -> GND
- ASM1 pad T21: GNDA -> GND
- ASM1 pad T4: GNDA -> GND
- ASM1 pad T5: GNDA -> GND
- ASM1 pad T6: VCCL -> unconnected-(ASM1E-VCCL-PadT6)
- ASM1 pad T8: VDD -> VDD095
- ASM1 pad T9: VDD -> VDD095
- ASM1 pad U1: GNDA -> GND
- ASM1 pad U11: VCCL -> unconnected-(ASM1E-VCCL-PadU11)
- ASM1 pad U13: VCCL -> unconnected-(ASM1E-VCCL-PadU13)
- ASM1 pad U14: VCCL -> unconnected-(ASM1E-VCCL-PadU14)
- ASM1 pad U16: VCCL -> unconnected-(ASM1E-VCCL-PadU16)
- ASM1 pad U17: GNDA -> GND
- ASM1 pad U18: GNDA -> GND
- ASM1 pad U2: GNDA -> GND
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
